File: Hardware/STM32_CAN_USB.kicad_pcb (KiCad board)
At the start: 2 copper layers, 49.7 x 36.5 mm, 28 parts, among them J1 USB_C_Receptacle_USB2.0_14P, J2 SWD, J3 CAN Connector, J4 JP1, SW1 RESET, U1 AP2112K-3.3, U2 STM32F103C8Tx, U3 SN65HVD230, Y1 8Mhz

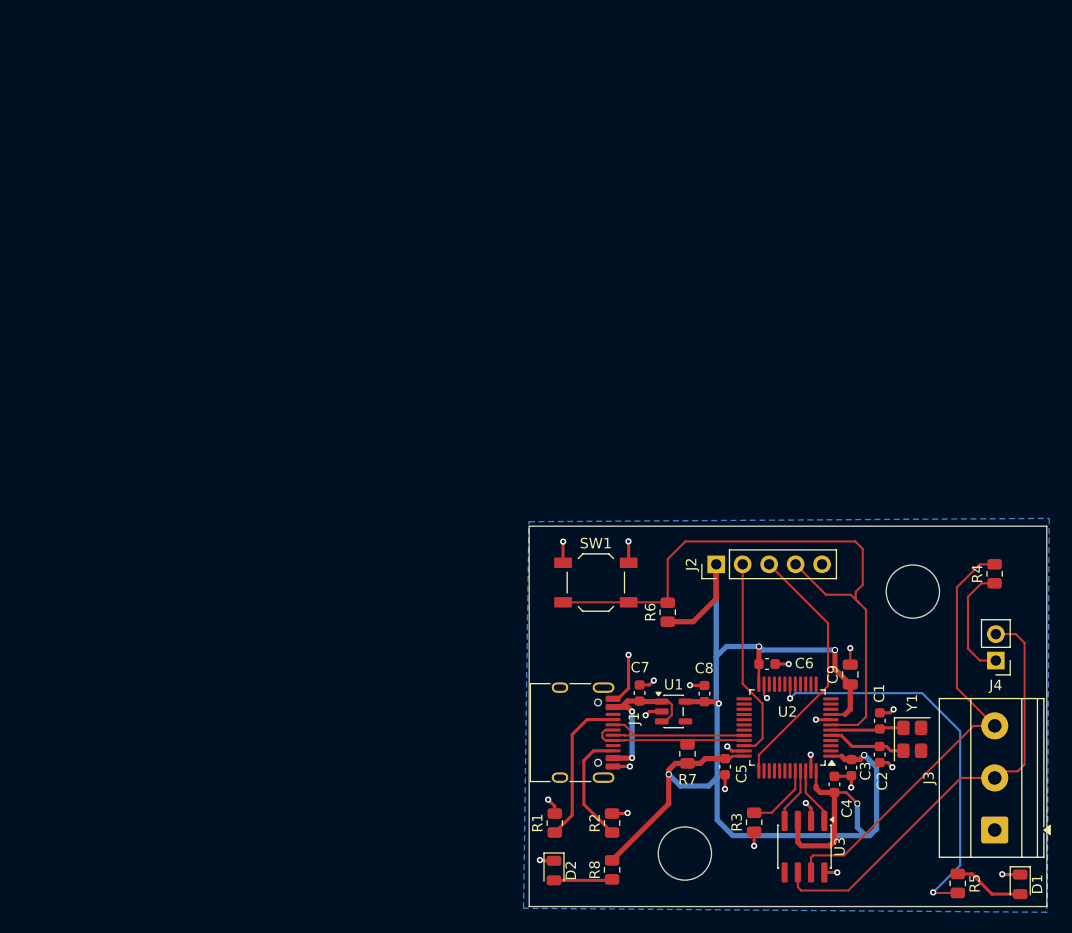
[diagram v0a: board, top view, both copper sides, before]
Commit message: Replace project with updated design
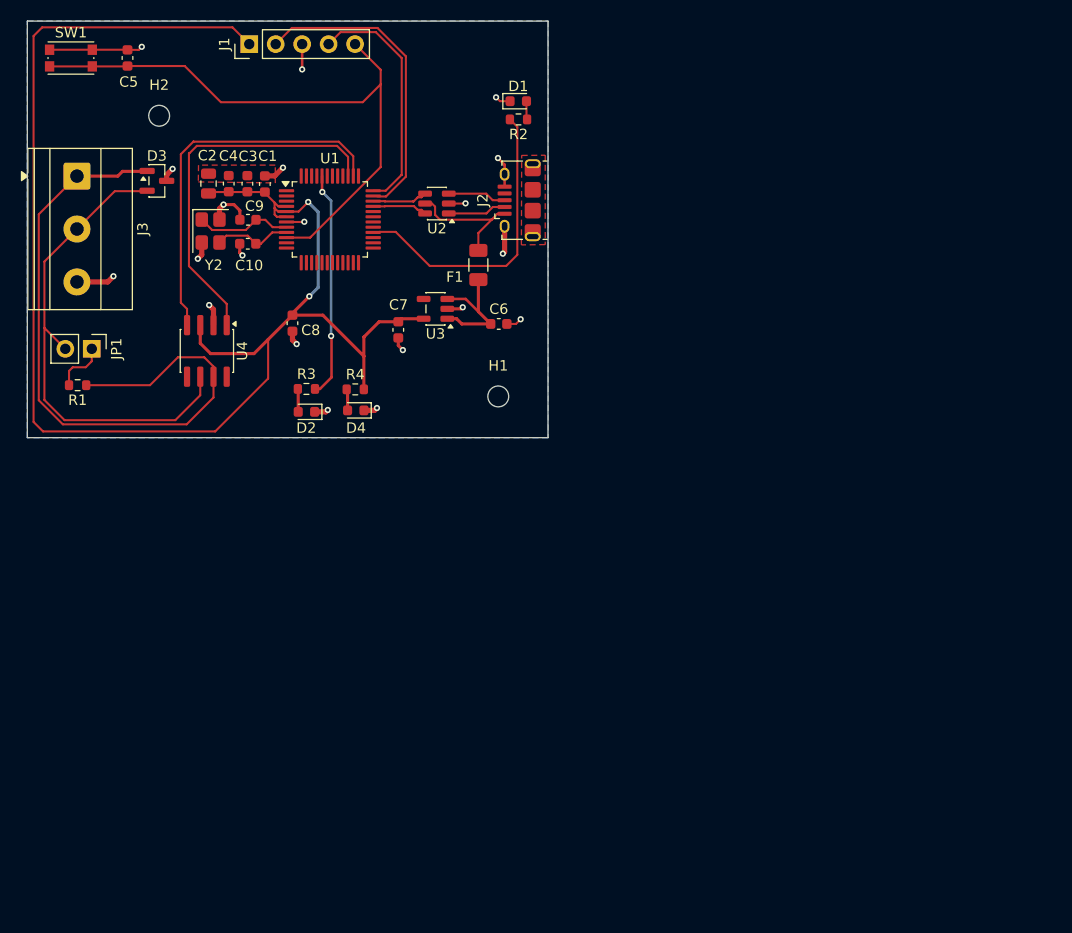
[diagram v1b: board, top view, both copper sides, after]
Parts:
- removed J4: JP1, Connector_PinHeader_2.54mm:PinHeader_1x02_P2.54mm_Vertical
- removed R5, R8: 330, Resistor_SMD:R_0805_2012Metric
- removed R6: 10K, Resistor_SMD:R_0805_2012Metric
- removed R7: 1.5K, Resistor_SMD:R_0805_2012Metric
- removed Y1: 8Mhz, Crystal:Crystal_SMD_3225-4Pin_3.2x2.5mm
- added C10: 5.6pF, Capacitor_SMD:C_0603_1608Metric, F.Cu at (99.5, 60.4)
- added D3: NUP2105L, Package_TO_SOT_SMD:SOT-23, F.Cu at (90.8, 54.3)
- added D4: LED_PWR, LED_SMD:LED_0603_1608Metric, F.Cu at (109.9, 76.4)
- added F1: Polyfuse, Fuse:Fuse_1206_3216Metric, F.Cu at (121.7, 62.4)
- added H1: MountingHole, MountingHole:MountingHole_2mm, F.Cu at (123.6, 75.0)
- added H2: MountingHole, MountingHole:MountingHole_2mm, F.Cu at (91.0, 48.1)
- added JP1: CAN_JP, Connector_PinHeader_2.54mm:PinHeader_1x02_P2.54mm_Vertical, F.Cu at (84.5, 70.5)
- added U4: TCAN332G, Package_SO:SOIC-8_3.9x4.9mm_P1.27mm, F.Cu at (95.6, 70.7)
- added Y2: 16Mhz, Crystal:Crystal_SMD_3225-4Pin_3.2x2.5mm, F.Cu at (96.0, 59.2)
- C1: value 22pF -> 100nF
- C2: value 22pF -> 4.7uF; footprint Capacitor_SMD:C_0603_1608Metric -> Capacitor_SMD:C_0805_2012Metric
- C4, C6: value 100nF -> 1uF
- C5: value 100nF -> 0.1uF
- C8: value 1uF -> 100nF
- C9: value 10uF -> 5.6pF; footprint Capacitor_SMD:C_0805_2012Metric -> Capacitor_SMD:C_0603_1608Metric
- D1: value CAN -> LED_USB; footprint LED_SMD:LED_0805_2012Metric -> LED_SMD:LED_0603_1608Metric
- D2: value PWR -> LED_CAN; footprint LED_SMD:LED_0805_2012Metric -> LED_SMD:LED_0603_1608Metric
- J1: value USB_C_Receptacle_USB2.0_14P -> SWD; footprint Connector_USB:USB_C_Receptacle_HRO_TYPE-C-31-M-12 -> Connector_PinHeader_2.54mm:PinHeader_1x05_P2.54mm_Vertical
- J2: value SWD -> USB_B_Micro; footprint Connector_PinHeader_2.54mm:PinHeader_1x05_P2.54mm_Vertical -> Connector_USB:USB_Micro-B_Amphenol_10118194_Horizontal
- J3: value CAN Connector -> CAN_Terminal; footprint TerminalBlock_Phoenix:TerminalBlock_Phoenix_MKDS-1,5-3_1x03_P5.00mm_Horizontal -> TerminalBlock_Phoenix:TerminalBlock_Phoenix_MKDS-1,5-3-5.08_1x03_P5.08mm_Horizontal
- R1: value 5.1K -> 120; footprint Resistor_SMD:R_0805_2012Metric -> Resistor_SMD:R_0603_1608Metric
- R2: value 5.1K -> 1K; footprint Resistor_SMD:R_0805_2012Metric -> Resistor_SMD:R_0603_1608Metric
- R3: value 10K -> 1K; footprint Resistor_SMD:R_0805_2012Metric -> Resistor_SMD:R_0603_1608Metric
- R4: value 120 -> 1K; footprint Resistor_SMD:R_0805_2012Metric -> Resistor_SMD:R_0603_1608Metric
- SW1: value RESET -> RESET_BUT; footprint Button_Switch_SMD:SW_SPST_TL3342 -> Button_Switch_SMD:SW_Push_1P1T_NO_CK_KMR2
- U1: value AP2112K-3.3 -> STM32G0B1CBTx; footprint Package_TO_SOT_SMD:SOT-23-5 -> Package_QFP:LQFP-48_7x7mm_P0.5mm
- U2: value STM32F103C8Tx -> USBLC6-2SC6; footprint Package_QFP:LQFP-48_7x7mm_P0.5mm -> Package_TO_SOT_SMD:SOT-23-6
- U3: value SN65HVD230 -> AP2112K-3.3; footprint Package_SO:SOIC-8_3.9x4.9mm_P1.27mm -> Package_TO_SOT_SMD:SOT-23-5
- moved J3 108.2 mm to (83.1, 53.9), turned to -90 degrees
- moved D1 89.3 mm to (125.5, 46.7), turned to 0 degrees
- moved C5 89.0 mm to (88.0, 42.5)
- moved C2 84.6 mm to (95.8, 54.6), turned to 90 degrees
- moved C4 81.9 mm to (97.7, 54.6), turned to 90 degrees
- moved C3 80.7 mm to (99.5, 54.6)
- moved C1 78.4 mm to (101.2, 54.6), turned to 90 degrees
- moved J1 73.0 mm to (99.7, 41.2), turned to 90 degrees
- moved C9 72.5 mm to (99.5, 58.1), turned to 180 degrees
- moved SW1 71.2 mm to (82.5, 42.5)
- moved R2 68.2 mm to (125.5, 48.4), turned to 180 degrees
- moved R4 63.9 mm to (109.8, 74.4), turned to 0 degrees
- moved U3 62.6 mm to (117.5, 66.6), turned to 180 degrees
- moved R1 62.2 mm to (83.2, 74.0), turned to 180 degrees
- moved U2 60.5 mm to (117.7, 56.5)
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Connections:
- C1 pad 1: GND -> +3V3
- C1 pad 2: Net-(U2-PD1) -> GND
- C2 pad 1: Net-(U2-PD0) -> +3V3
- C3 pad 1: GND -> +3V3
- C3 pad 2: +3.3V -> GND
- C4 pad 1: GND -> +3V3
- C4 pad 2: +3.3V -> GND
- C5 pad 1: GND -> /RESET
- C5 pad 2: +3.3V -> GND
- C6 pad 1: GND -> Net-(U3-EN)
- C6 pad 2: +3.3V -> GND
- C7 pad 1: GND -> +3V3
- C7 pad 2: Net-(U1-EN) -> GND
- C8 pad 1: GND -> +3V3
- C8 pad 2: +3.3V -> GND
- C9 pad 1: +3.3V -> Net-(U1-PF0)
- J2 pad 1: +3.3V -> /VBUS
- J2 pad 2: /SWDIO -> Net-(J2-D-)
- J2 pad 3: /SWCLK -> Net-(J2-D+)
- J2 pad 4: /NRST -> unconnected-(J2-ID-Pad4)
- J3 pad 1: GND -> /CAN_H
- J3 pad 2: Net-(J3-Pin_2) -> /CAN_L
- J3 pad 3: Net-(J3-Pin_3) -> GND
- R1 pad 1: Net-(J1-CC1) -> /CAN_H
- R1 pad 2: GND -> Net-(JP1-A)
- R2 pad 1: Net-(J1-CC2) -> Net-(D1-A)
- R2 pad 2: GND -> /USB_LED
- R3 pad 1: GND -> Net-(D2-A)
- R3 pad 2: Net-(U2-BOOT0) -> /CAN_LED
- R4 pad 2: Net-(J3-Pin_3) -> +3V3
- SW1 pad 2: /NRST -> /RESET
- U1 pad 1: Net-(U1-EN) -> unconnected-(U1-PC13-Pad1)
- U1 pad 2: GND -> unconnected-(U1-PC14-Pad2)
- U1 pad 3: Net-(U1-EN) -> unconnected-(U1-PC15-Pad3)
- U1 pad 4: unconnected-(U1-NC-Pad4) -> +3V3
- U1 pad 5: +3.3V -> +3V3
- U2 pad 1: +3.3V -> Net-(J2-D-)
- U2 pad 2: unconnected-(U2-PC13-Pad2) -> GND
- U2 pad 3: unconnected-(U2-PC14-Pad3) -> Net-(J2-D+)
- U2 pad 4: unconnected-(U2-PC15-Pad4) -> /USB_DP
- U2 pad 5: Net-(U2-PD0) -> /VBUS
- U2 pad 6: Net-(U2-PD1) -> /USB_DN
- U3 pad 1: /CAN_TX -> Net-(U3-EN)
- U3 pad 3: +3.3V -> Net-(U3-EN)
- U3 pad 4: /CAN_RX -> unconnected-(U3-NC-Pad4)
- U3 pad 5: unconnected-(U3-Vref-Pad5) -> +3V3
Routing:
- net +3V3: track 0.00 -> 146.7 mm, vias 0 -> 2
- net +3.3V: track 132.9 -> 0.00 mm, vias 6 -> 0
- net /CAN_H: track 0.00 -> 66.2 mm
- net /NRST: track 62.0 -> 0.00 mm
- net /RESET: track 0.00 -> 58.6 mm
- net /CAN_L: track 0.00 -> 47.6 mm
- net Net-(J3-Pin_3): track 43.7 -> 0.00 mm
- net Net-(J3-Pin_2): track 43.1 -> 0.00 mm
- net /FDCAN1_RX: track 0.00 -> 36.2 mm
- net /FDCAN1_TX: track 0.00 -> 35.8 mm
- net /USB_LED: track 0.00 -> 28.4 mm
- net /CAN_LED: track 38.4 -> 21.8 mm
- net Net-(U1-EN): track 16.5 -> 0.00 mm, vias 2 -> 0
- net /USB+: track 15.7 -> 0.00 mm
- net /USB-: track 15.5 -> 0.00 mm
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- added copper zone on F.Cu, net GND
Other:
- board size 49.7 x 36.5 mm -> 50 x 40 mm
